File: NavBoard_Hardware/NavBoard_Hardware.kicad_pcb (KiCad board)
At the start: 2 copper layers, 61 x 100 mm, 52 parts, among them J1 Conn_Coaxial, U2 ATMEGA328P-Project_Library, U3 OKI, U4 OKI, U5 FGPMMOPA6H, Y1 Crystal

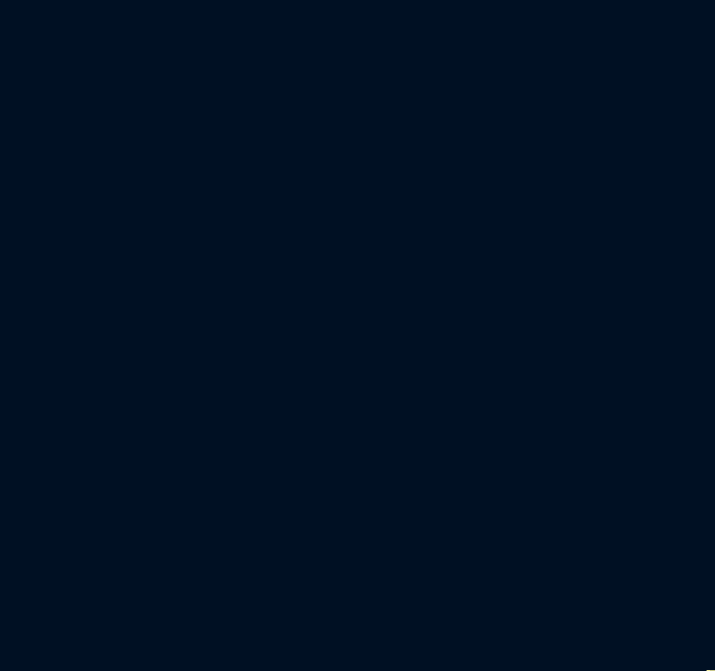
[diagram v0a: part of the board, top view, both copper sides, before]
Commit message: saved
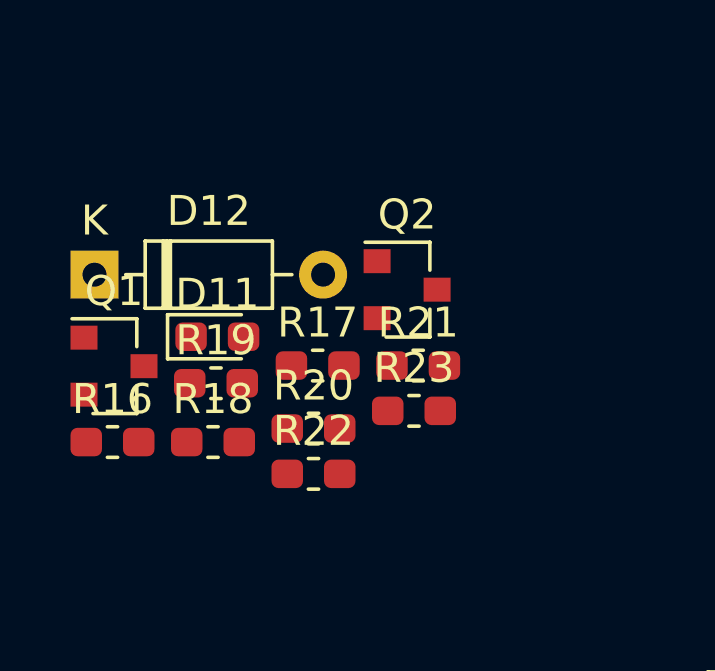
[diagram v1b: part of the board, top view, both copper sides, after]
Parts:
- added D11: LED, LED_SMD:LED_0603_1608Metric_Pad1.05x0.95mm_HandSolder, F.Cu at (91.5, 74.5)
- added D12: 1N4148, Diode_THT:D_DO-35_SOD27_P7.62mm_Horizontal, F.Cu at (87.4, 72.4)
- added Q1: BSS138, Package_TO_SOT_SMD:SOT-23, F.Cu at (88.1, 75.4)
- added Q2: BSS138, Package_TO_SOT_SMD:SOT-23, F.Cu at (97.9, 72.9)
- added R16: 500, Resistor_SMD:R_0603_1608Metric_Pad1.05x0.95mm_HandSolder, F.Cu at (88.0, 78.0)
- added R17: 10K, Resistor_SMD:R_0603_1608Metric_Pad1.05x0.95mm_HandSolder, F.Cu at (94.9, 75.4)
- added R18: 10K, Resistor_SMD:R_0603_1608Metric_Pad1.05x0.95mm_HandSolder, F.Cu at (91.4, 78.0)
- added R19: 10K, Resistor_SMD:R_0603_1608Metric_Pad1.05x0.95mm_HandSolder, F.Cu at (91.5, 76.0)
- added R20: 10K, Resistor_SMD:R_0603_1608Metric_Pad1.05x0.95mm_HandSolder, F.Cu at (94.7, 77.5)
- added R21: 10K, Resistor_SMD:R_0603_1608Metric_Pad1.05x0.95mm_HandSolder, F.Cu at (98.2, 75.4)
- added R22: 30K, Resistor_SMD:R_0603_1608Metric_Pad1.05x0.95mm_HandSolder, F.Cu at (94.7, 79.0)
- added R23: 0, Resistor_SMD:R_0603_1608Metric_Pad1.05x0.95mm_HandSolder, F.Cu at (98.1, 76.9)
- Conn4: value Molex_SL_04-MRDT_Connectors -> Molex_SL_04
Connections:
- C1 pad 1: +3V3 -> +5V
- R2 pad 1: +3V3 -> +5V
- R5 pad 1: Programming_TX -> Programming_RX
- R6 pad 1: Programming_RX -> Programming_TX
- U1 pad PA6: Net-(U1-PadPA6) -> TIVA_RX
- U1 pad PC7: IMU_TX -> TIVA_TX
- U1 pad PL0: LIDAR_SDA -> Net-(U1-PadPL0)
- U1 pad PL1: LIDAR_SCL -> Net-(U1-PadPL1)
- U2 pad 20: +3V3 -> +5V
- U2 pad 4: Net-(U2-Pad4) -> TIVAtoATM_RX
- U2 pad 5: Net-(U2-Pad5) -> TIVAtoATM_TX
- U2 pad 7: +3V3 -> +5V
